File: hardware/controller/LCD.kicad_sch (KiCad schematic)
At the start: 1 part, among them U101 3.2inch_IPS_SPI_Module_ILI9341

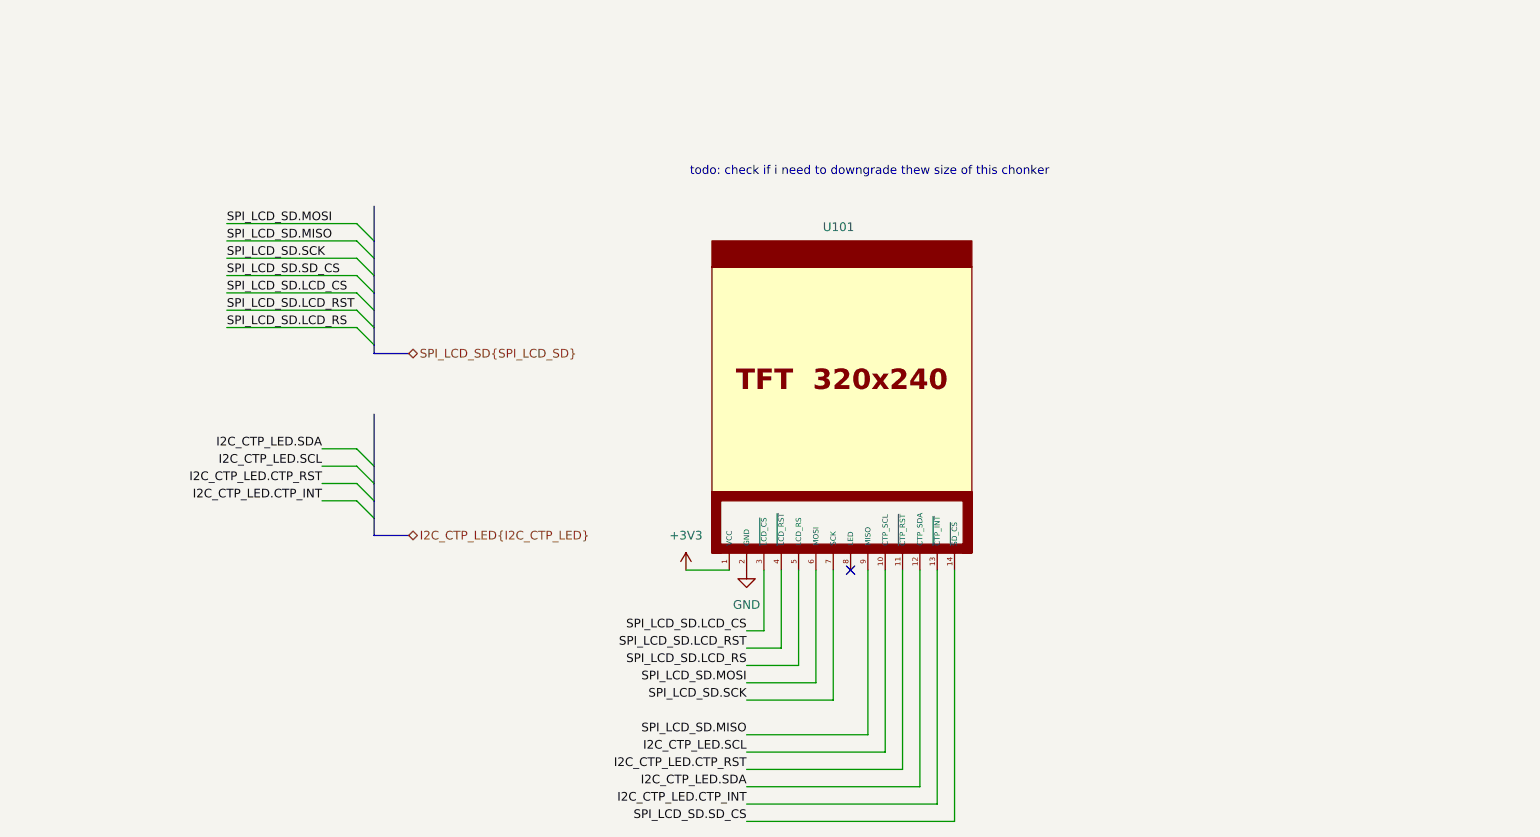
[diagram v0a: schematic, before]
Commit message: forgor
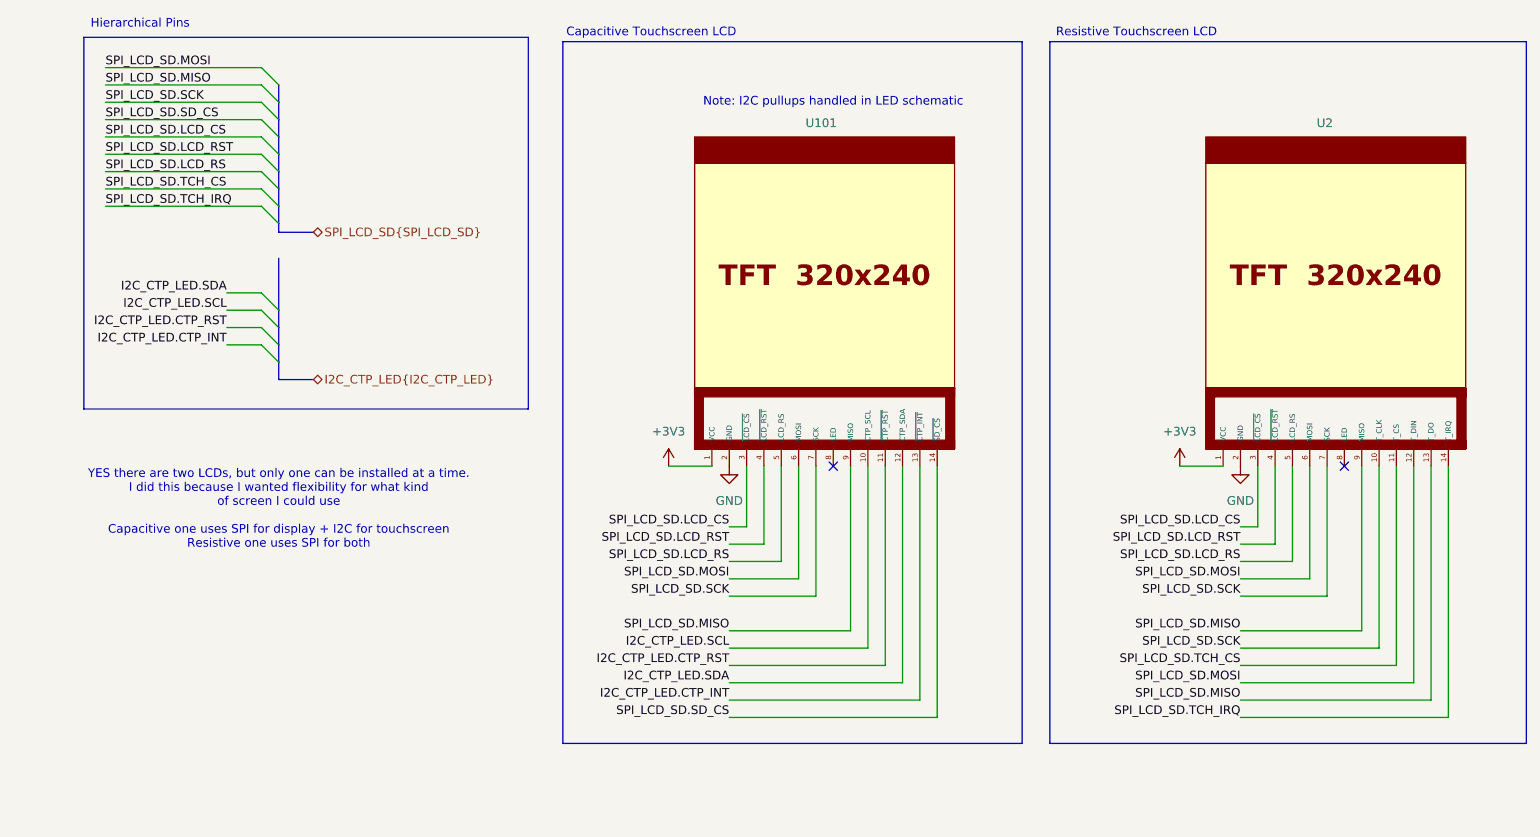
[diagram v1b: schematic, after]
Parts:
- added U2: 3.2inch_IPS_SPI_Module_ILI9341, SamacSys_Parts:TFT-320x240, symbol SamacSys_Parts:2.4inch_IPS_SPI_Module_ILI9341
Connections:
- net +3V3: now also U2.1 (VCC)
- net GND: now also U2.2 (GND)
- net SPI_LCD_SD.LCD_CS: now also U2.3 (~{LCD_CS})
- net SPI_LCD_SD.LCD_RS: now also U2.5 (LCD_RS)
- net SPI_LCD_SD.LCD_RST: now also U2.4 (~{LCD_RST})
- net SPI_LCD_SD.MISO: now also U2.13 (T_DO), U2.9 (MISO)
- net SPI_LCD_SD.MOSI: now also U2.12 (T_DIN), U2.6 (MOSI)
- net SPI_LCD_SD.SCK: now also U2.10 (T_CLK), U2.7 (SCK)
- new net SPI_LCD_SD.TCH_CS: U2.11 (T_CS)
- new net SPI_LCD_SD.TCH_IRQ: U2.14 (T_IRQ)
- no-connect marks 1 -> 2
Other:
- note added: "Capacitive Touchscreen LCD"
- note added: "Hierarchical Pins"
- note added: "Note: I2C pullups handled in LED schematic"
- note added: "Resistive Touchscreen LCD"
- note added: "YES there are two LCDs, but only one can be installed at a time. I did this because I wanted flexibility for what kind of screen I could use Capacitive one uses SPI for display + I2C for touchscreen Resistive one uses SPI for both"
- note removed: "todo: check if i need to downgrade thew size of this chonker"
- moved on the sheet: U101
